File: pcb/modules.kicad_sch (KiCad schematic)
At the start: 12 parts, among them IC2 E22-900M22S, J2 Conn_01x08_Pin, J3 Conn_Coaxial, J4 Conn_Coaxial, U4 BME280, U6 NEO-M8M

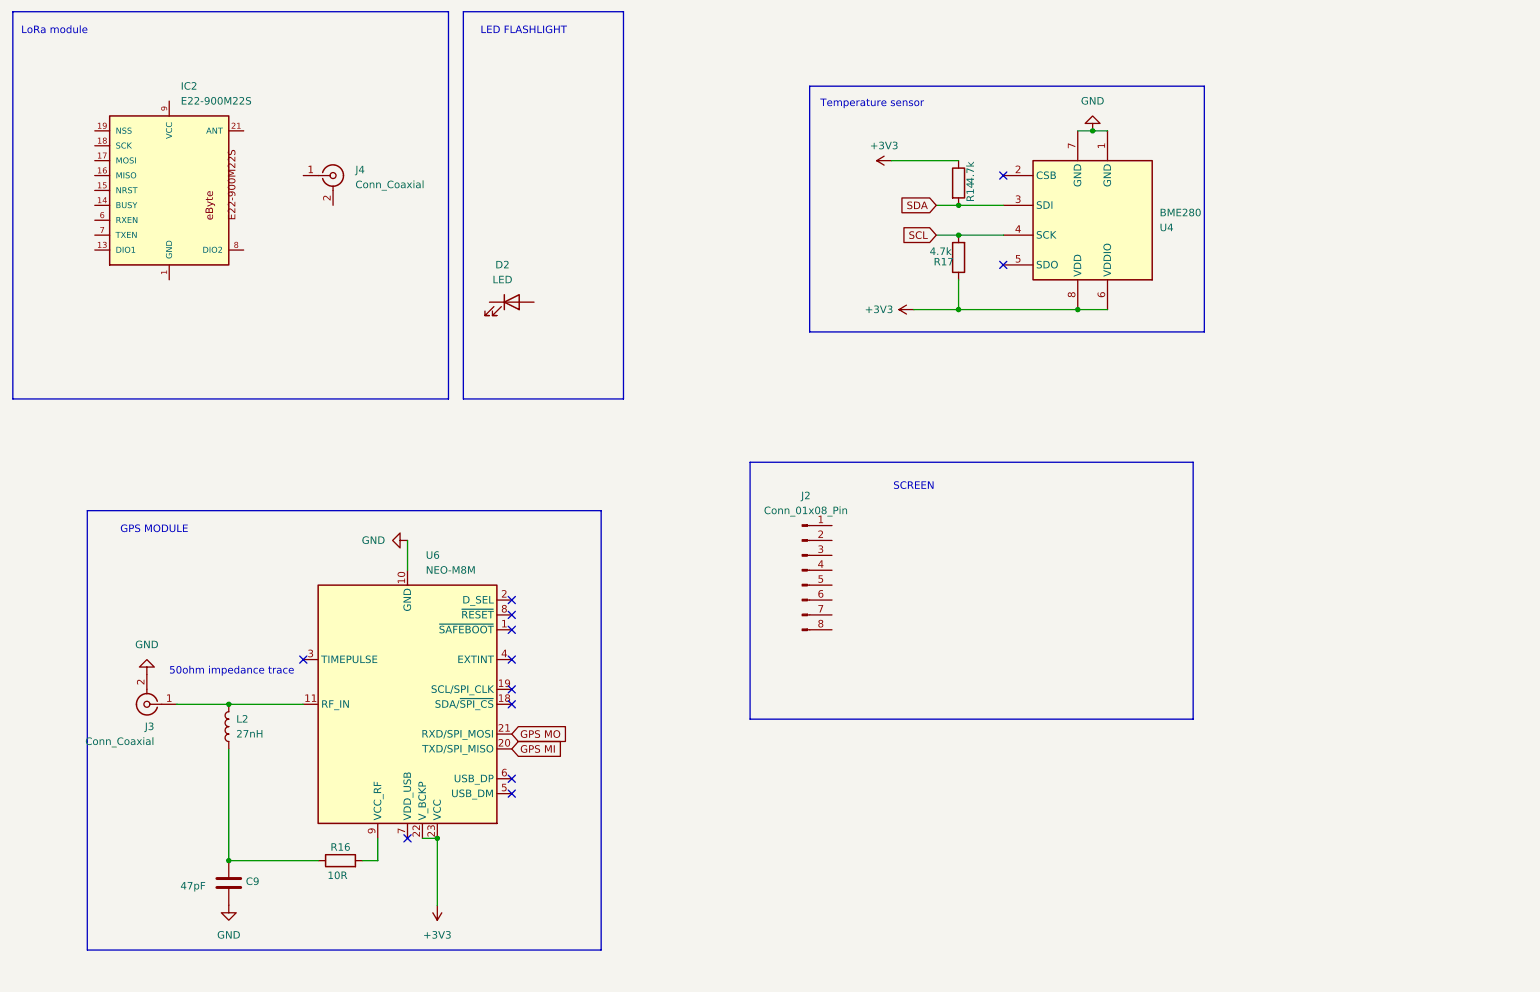
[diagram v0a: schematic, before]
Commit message: Updating schematic & pcb & BOM
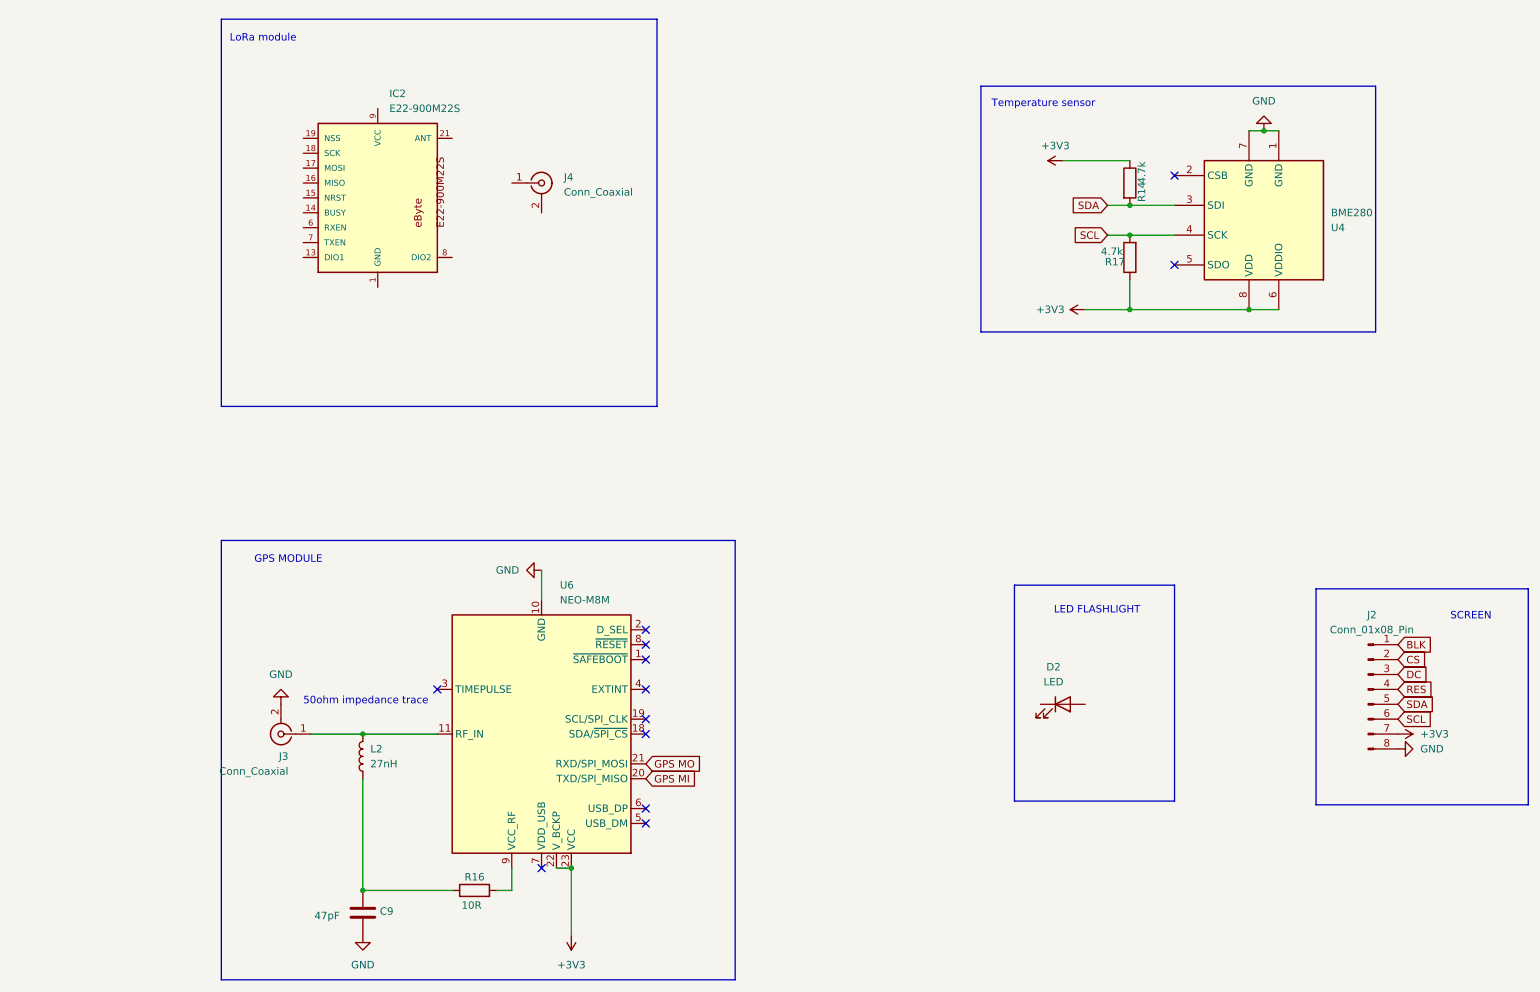
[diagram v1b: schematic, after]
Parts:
- J3: footprint (none) -> Connector_Coaxial:U.FL_Hirose_U.FL-R-SMT-1_Vertical
- L2: footprint (none) -> Inductor_SMD:L_0805_2012Metric
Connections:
- net +3V3: now also J2.7 (Pin_7)
- net GND: now also J2.8 (Pin_8)
- net SCL: now also J2.6 (Pin_6)
- net SDA: now also J2.5 (Pin_5)
- net BLK: now reaches J2.1 (Pin_1)
- net CS: now reaches J2.2 (Pin_2)
- net DC: now reaches J2.3 (Pin_3)
- net RES: now reaches J2.4 (Pin_4)
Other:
- title: (none) -> NOMAD MODULES
- moved on the sheet: C9, D2, IC2, J2, J3, J4, L2, R14, R16, R17, U4, U6
